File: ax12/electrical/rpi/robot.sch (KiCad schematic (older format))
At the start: 23 parts, among them J1 Raspberry_Pi_2_3, J2 IMU, J3 Lidar, J4 I2C, J5 SPI, J6 Pi USB Pwr, J7 Audio, J8 SERIAL, J9 PWR BOARD, Q1 BSS138, U1 AP1117-50, U2 74LVC1G125, U3 74LVC1G126

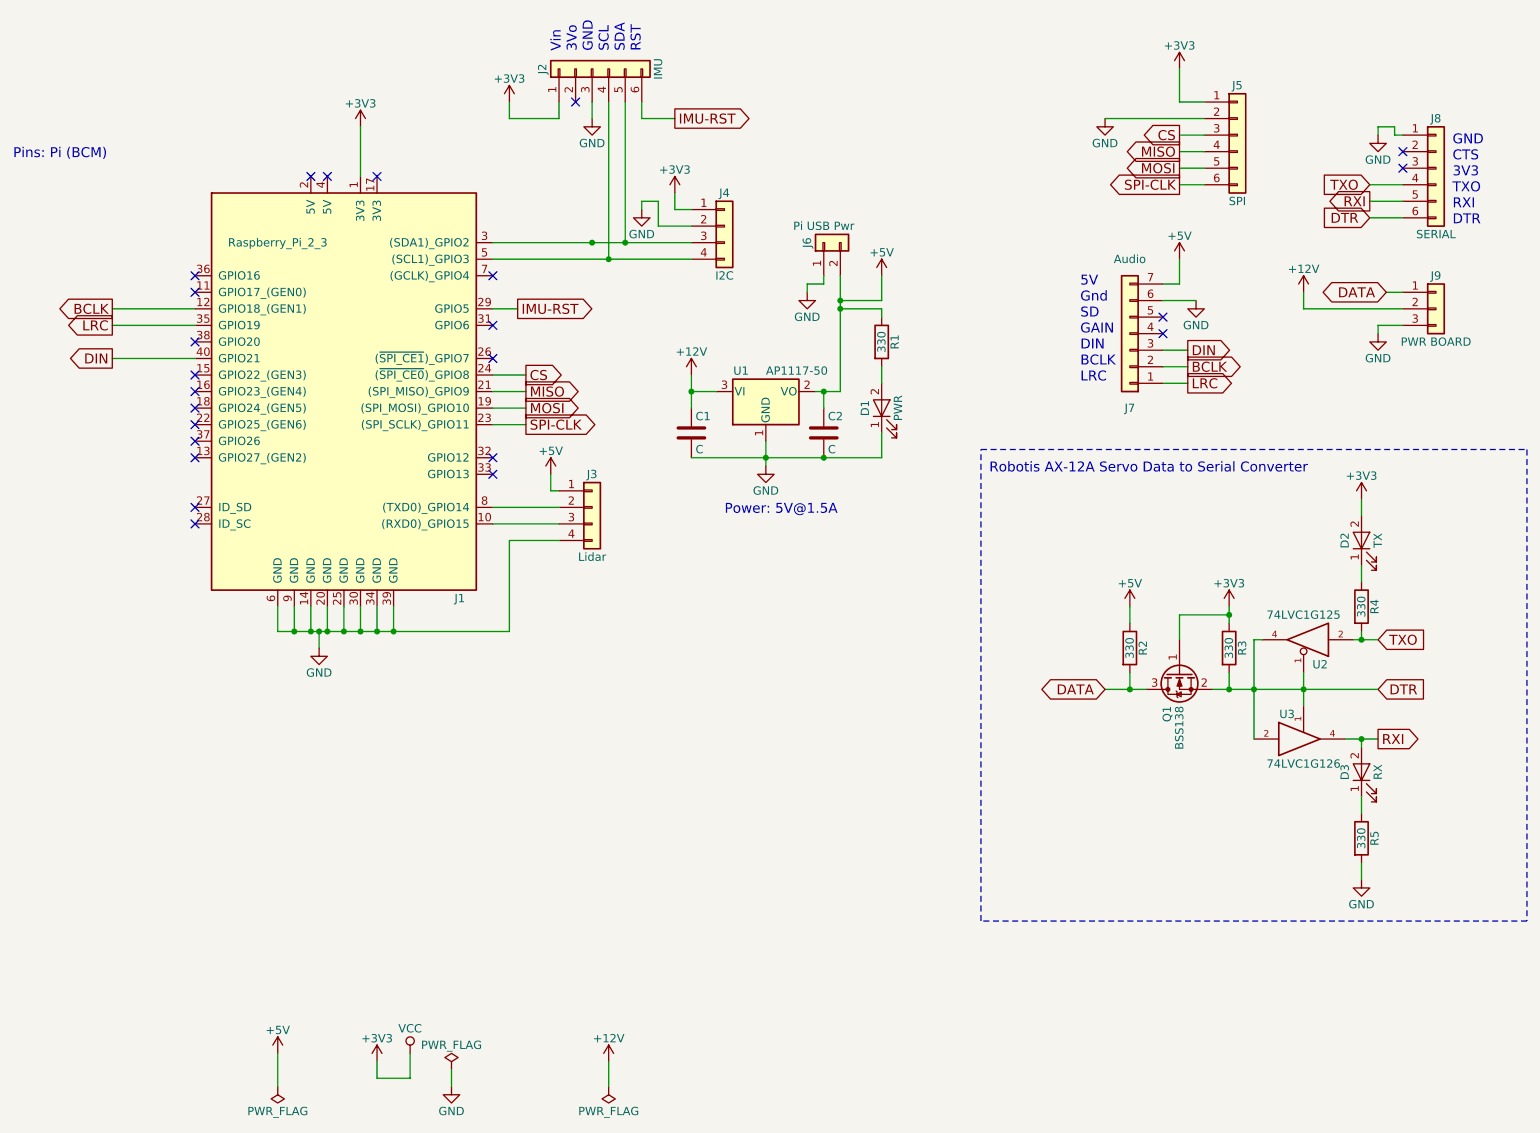
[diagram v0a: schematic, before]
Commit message: power 3 done :tada: :electric_plug:
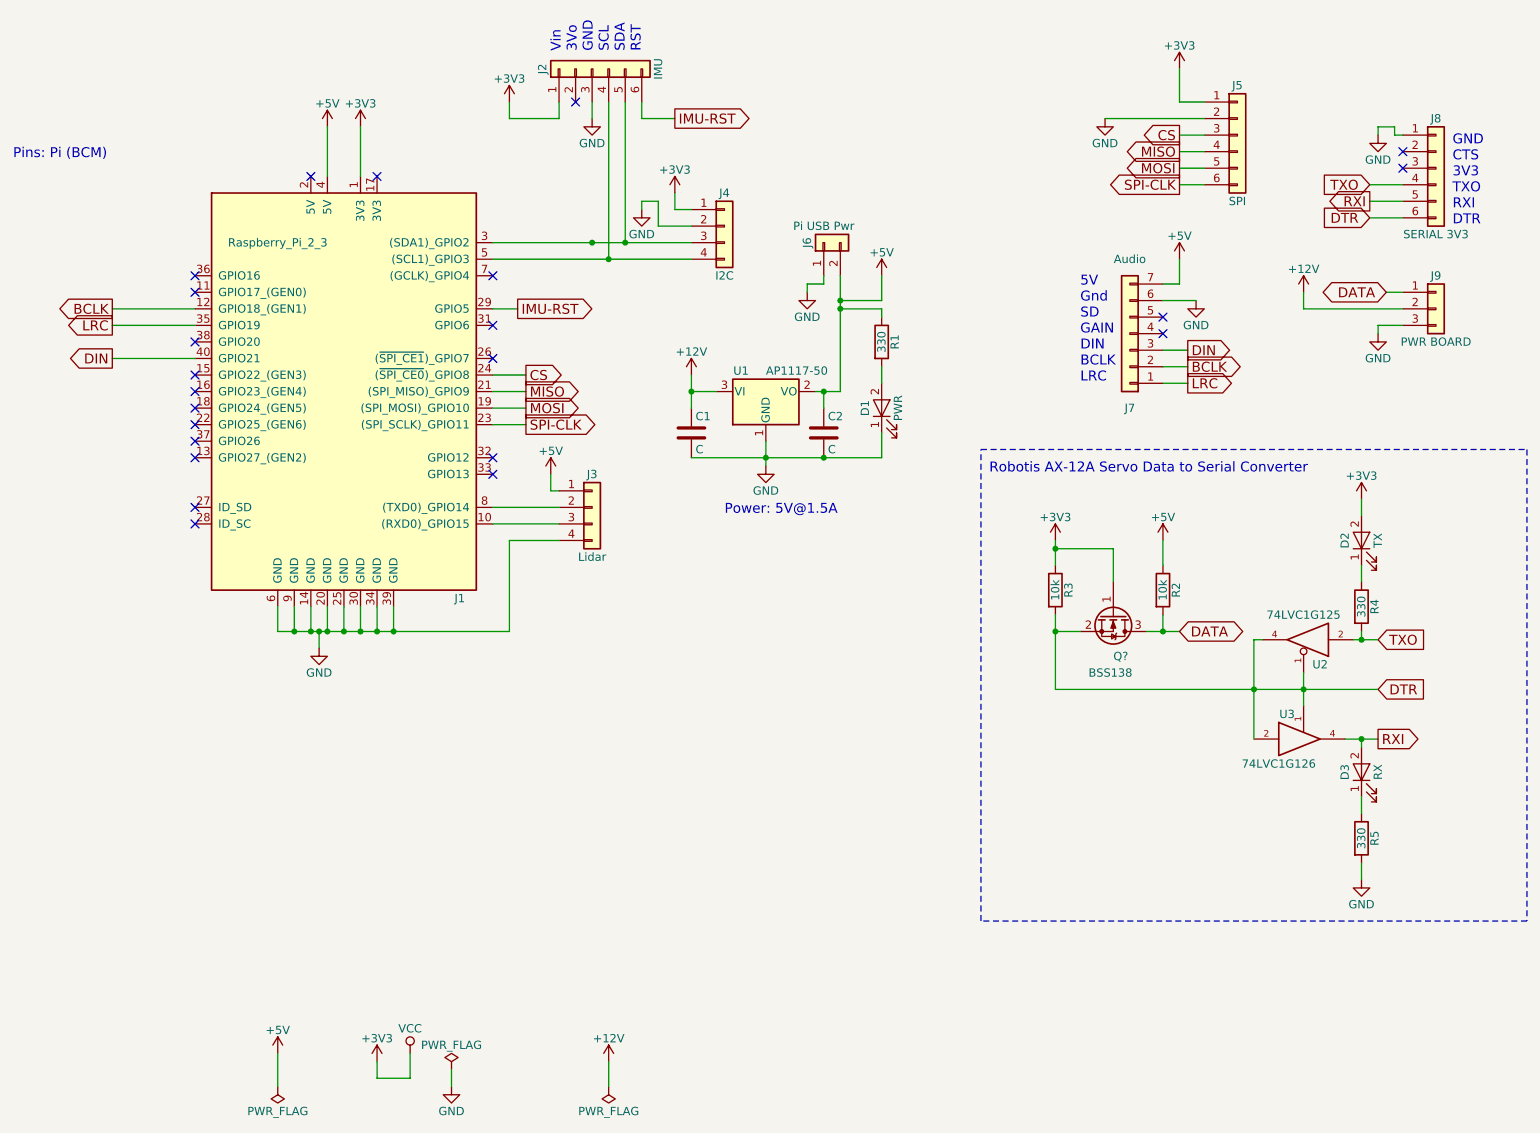
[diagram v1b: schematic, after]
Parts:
- removed Q1: BSS138, TO_SOT_Packages_SMD:SOT-23, symbol BSS138
- added Q?: BSS138, TO_SOT_Packages_SMD:SOT-23, symbol BSS138
- J8: value SERIAL -> SERIAL 3V3
- R2, R3: value 330 -> 10k
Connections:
- net +3V3: now also Q?.1 (G)
- net +5V: now also J1.4 (5V)
- net DATA: now also Q?.3 (D)
- net DTR: now also Q?.2 (S)
- no-connect marks 24 -> 23
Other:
- moved on the sheet: R2, R3
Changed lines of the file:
@@
 $EndComp
 NoConn ~ 3300 1650
-NoConn ~ 3400 1650
 $Comp
 L +3V3 #PWR016
@@
 P 9300 5050
 F 0 "U3" H 9200 5200 50  0000 C CNN
-F 1 "74LVC1G126" H 9300 4900 50  0000 C CNN
+F 1 "74LVC1G126" H 9150 4900 50  0000 C CNN
 F 2 "TO_SOT_Packages_SMD:SOT-23-5_HandSoldering" H 9300 5050 50  0001 C CNN
 F 3 "" H 9300 5050 50  0001 C CNN
@@
 $EndComp
 $Comp
-L BSS138 Q1
-U 1 1 5AA2CE83
-P 8550 4650
-F 0 "Q1" H 8750 4725 50  0000 L CNN
-F 1 "BSS138" H 8750 4650 50  0000 L CNN
-F 2 "TO_SOT_Packages_SMD:SOT-23" H 8750 4575 50  0001 L CIN
-F 3 "" H 8550 4650 50  0001 L CNN
-	1    8550 4650
-	0    -1   1    0
-$EndComp
-$Comp
 L R R3
 U 1 1 5AA2CFAD
-P 8850 4500
-F 0 "R3" V 8930 4500 50  0000 C CNN
-F 1 "330" V 8850 4500 50  0000 C CNN
-F 2 "Resistors_SMD:R_1206_HandSoldering" V 8780 4500 50  0001 C CNN
-F 3 "" H 8850 4500 50  0001 C CNN
-	1    8850 4500
+P 7800 4150
+F 0 "R3" V 7880 4150 50  0000 C CNN
+F 1 "10k" V 7800 4150 50  0000 C CNN
+F 2 "Resistors_SMD:R_1206_HandSoldering" V 7730 4150 50  0001 C CNN
+F 3 "" H 7800 4150 50  0001 C CNN
+	1    7800 4150
 	1    0    0    -1
 $EndComp
@@
 L R R2
 U 1 1 5AA2CFFB
-P 8250 4500
-F 0 "R2" V 8330 4500 50  0000 C CNN
-F 1 "330" V 8250 4500 50  0000 C CNN
-F 2 "Resistors_SMD:R_1206_HandSoldering" V 8180 4500 50  0001 C CNN
-F 3 "" H 8250 4500 50  0001 C CNN
-	1    8250 4500
+P 8450 4150
+F 0 "R2" V 8530 4150 50  0000 C CNN
+F 1 "10k" V 8450 4150 50  0000 C CNN
+F 2 "Resistors_SMD:R_1206_HandSoldering" V 8380 4150 50  0001 C CNN
+F 3 "" H 8450 4150 50  0001 C CNN
+	1    8450 4150
 	1    0    0    -1
 $EndComp
@@
 L +5V #PWR021
 U 1 1 5AA2D056
-P 8250 4250
-F 0 "#PWR021" H 8250 4100 50  0001 C CNN
-F 1 "+5V" H 8250 4390 50  0000 C CNN
-F 2 "" H 8250 4250 50  0001 C CNN
-F 3 "" H 8250 4250 50  0001 C CNN
-	1    8250 4250
+P 8450 3850
+F 0 "#PWR021" H 8450 3700 50  0001 C CNN
+F 1 "+5V" H 8450 3990 50  0000 C CNN
+F 2 "" H 8450 3850 50  0001 C CNN
+F 3 "" H 8450 3850 50  0001 C CNN
+	1    8450 3850
 	1    0    0    -1
 $EndComp
@@
 L +3V3 #PWR022
 U 1 1 5AA2DAAC
-P 8850 4250
-F 0 "#PWR022" H 8850 4100 50  0001 C CNN
-F 1 "+3V3" H 8850 4390 50  0000 C CNN
-F 2 "" H 8850 4250 50  0001 C CNN
-F 3 "" H 8850 4250 50  0001 C CNN
-	1    8850 4250
-	1    0    0    -1
-$EndComp
-Text GLabel 8100 4750 0    60   BiDi ~ 0
+P 7800 3850
+F 0 "#PWR022" H 7800 3700 50  0001 C CNN
+F 1 "+3V3" H 7800 3990 50  0000 C CNN
+F 2 "" H 7800 3850 50  0001 C CNN
+F 3 "" H 7800 3850 50  0001 C CNN
+	1    7800 3850
+	1    0    0    -1
+$EndComp
+Text GLabel 8550 4400 2    60   BiDi ~ 0
 DATA
 Text GLabel 9750 4450 2    60   Input ~ 0
@@
 P 10100 1600
 F 0 "J8" H 10100 1900 50  0000 C CNN
-F 1 "SERIAL" H 10100 1200 50  0000 C CNN
+F 1 "SERIAL 3V3" H 10100 1200 50  0000 C CNN
 F 2 "Pin_Headers:Pin_Header_Straight_1x06_Pitch2.54mm" H 10100 1600 50  0001 C CNN
 F 3 "" H 10100 1600 50  0001 C CNN
@@
 	9600 4450 9750 4450
 Wire Wire Line
-	8750 4750 9750 4750
-Wire Wire Line
 	9300 4650 9300 4850
 Connection ~ 9300 4750
 Wire Wire Line
-	8850 4650 8850 4750
-Connection ~ 8850 4750
-Wire Wire Line
-	8850 4250 8850 4350
-Wire Wire Line
-	8250 4250 8250 4350
-Wire Wire Line
-	8100 4750 8350 4750
-Wire Wire Line
 	9050 4450 9000 4450
 Wire Wire Line
@@
 Wire Wire Line
 	9550 5050 9750 5050
-Wire Wire Line
-	8250 4650 8250 4750
-Connection ~ 8250 4750
-Wire Wire Line
-	8550 4450 8550 4300
-Wire Wire Line
-	8550 4300 8850 4300
-Connection ~ 8850 4300
 Wire Wire Line
 	3100 6950 3100 7150
@@
 Text Notes 5800 3700 0    60   ~ 0
 Power: 5V@1.5A
+$Comp
+L BSS138 Q?
+U 1 1 5AAD3B03
+P 8150 4300
+F 0 "Q?" V 8400 4300 50  0000 L CNN
+F 1 "BSS138" V 8500 4150 50  0000 L CNN
+F 2 "TO_SOT_Packages_SMD:SOT-23" H 8350 4225 50  0001 L CIN
+F 3 "" H 8150 4300 50  0001 L CNN
+	1    8150 4300
+	0    1    1    0
+$EndComp
+Wire Wire Line
+	8350 4400 8550 4400
+Wire Wire Line
+	8450 4300 8450 4400
+Connection ~ 8450 4400
+Wire Wire Line
+	8450 4000 8450 3850
+Wire Wire Line
+	7800 4000 7800 3850
+Wire Wire Line
+	8150 4100 8150 3900
+Wire Wire Line
+	8150 3900 7800 3900
+Connection ~ 7800 3900
+Wire Wire Line
+	7800 4300 7800 4750
+Wire Wire Line
+	7800 4400 7950 4400
+Wire Wire Line
+	7800 4750 9750 4750
+Connection ~ 7800 4400
+$Comp
+L +5V #PWR?
+U 1 1 5AAD5DA7
+P 3400 1350
+F 0 "#PWR?" H 3400 1200 50  0001 C CNN
+F 1 "+5V" H 3400 1490 50  0000 C CNN
+F 2 "" H 3400 1350 50  0001 C CNN
+F 3 "" H 3400 1350 50  0001 C CNN
+	1    3400 1350
+	1    0    0    -1
+$EndComp
+Wire Wire Line
+	3400 1650 3400 1350
 $EndSCHEMATC
